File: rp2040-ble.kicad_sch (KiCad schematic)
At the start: 41 parts, among them J1 Conn_01x15, J2 Conn_01x15, J3 USB_B_Micro, J4 Conn_01x03, SW1 SW_Push, SW2 SW_Push, U1 RP2040, U2 W25Q128JVS, U3 HM-BT4502, U4 NCP1117DT33G, Y1 ABLS-12.000MHZ-B4-T

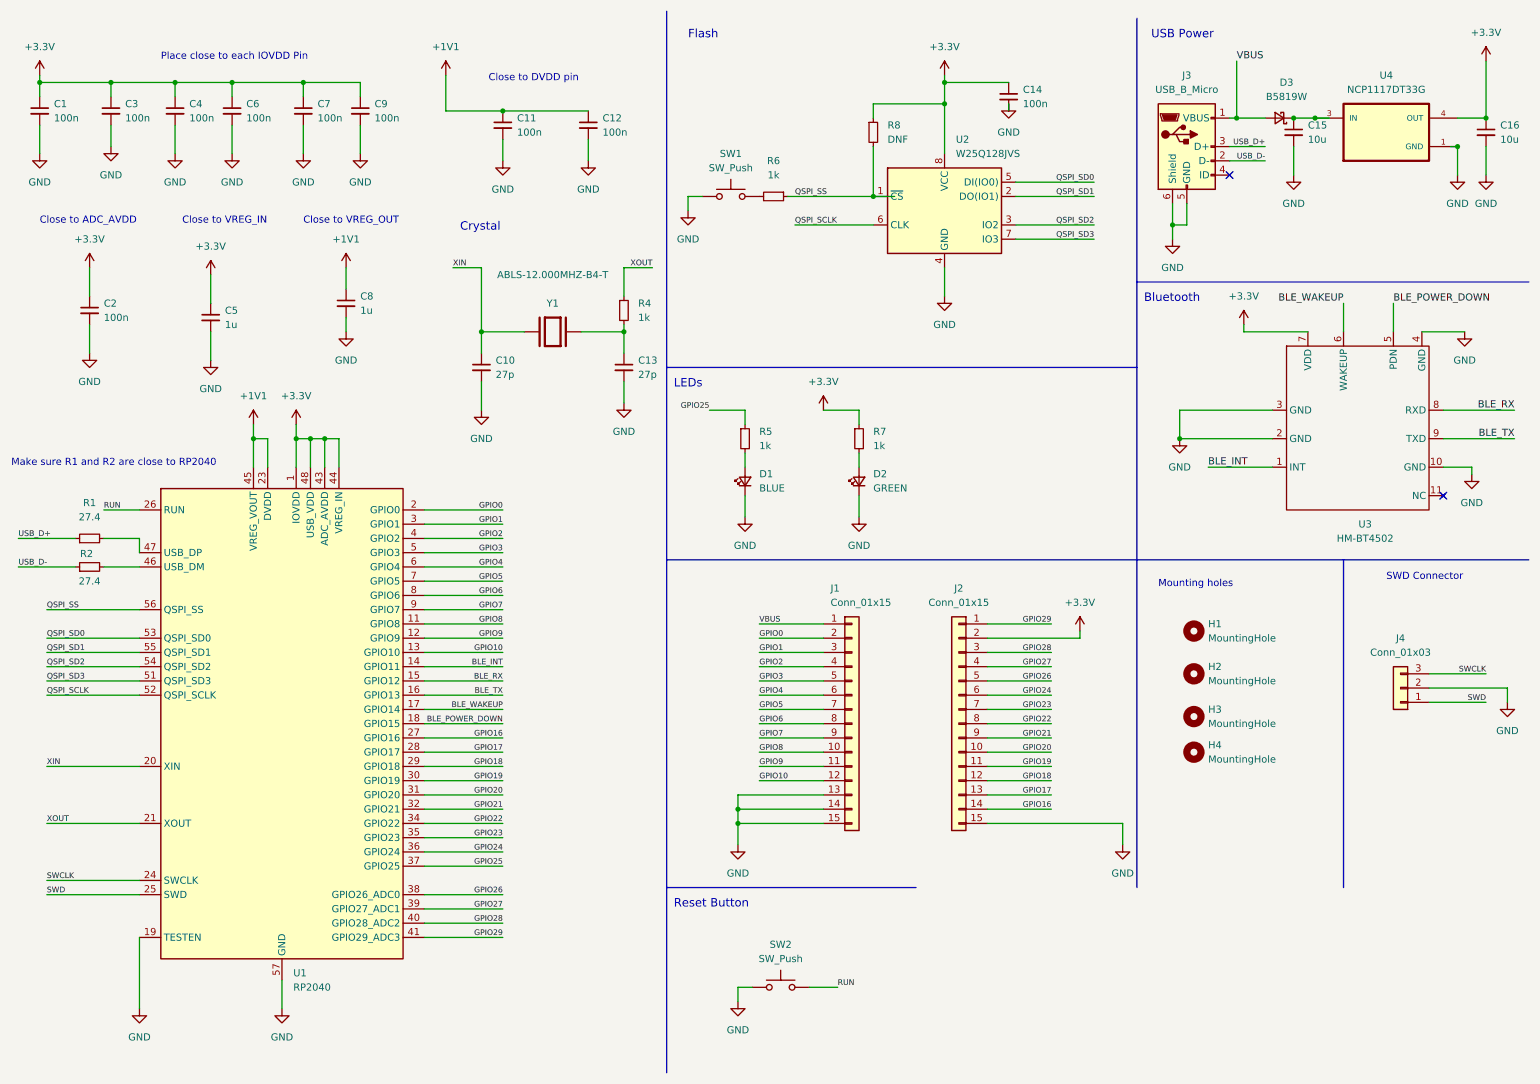
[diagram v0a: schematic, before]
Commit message: PCB roouting
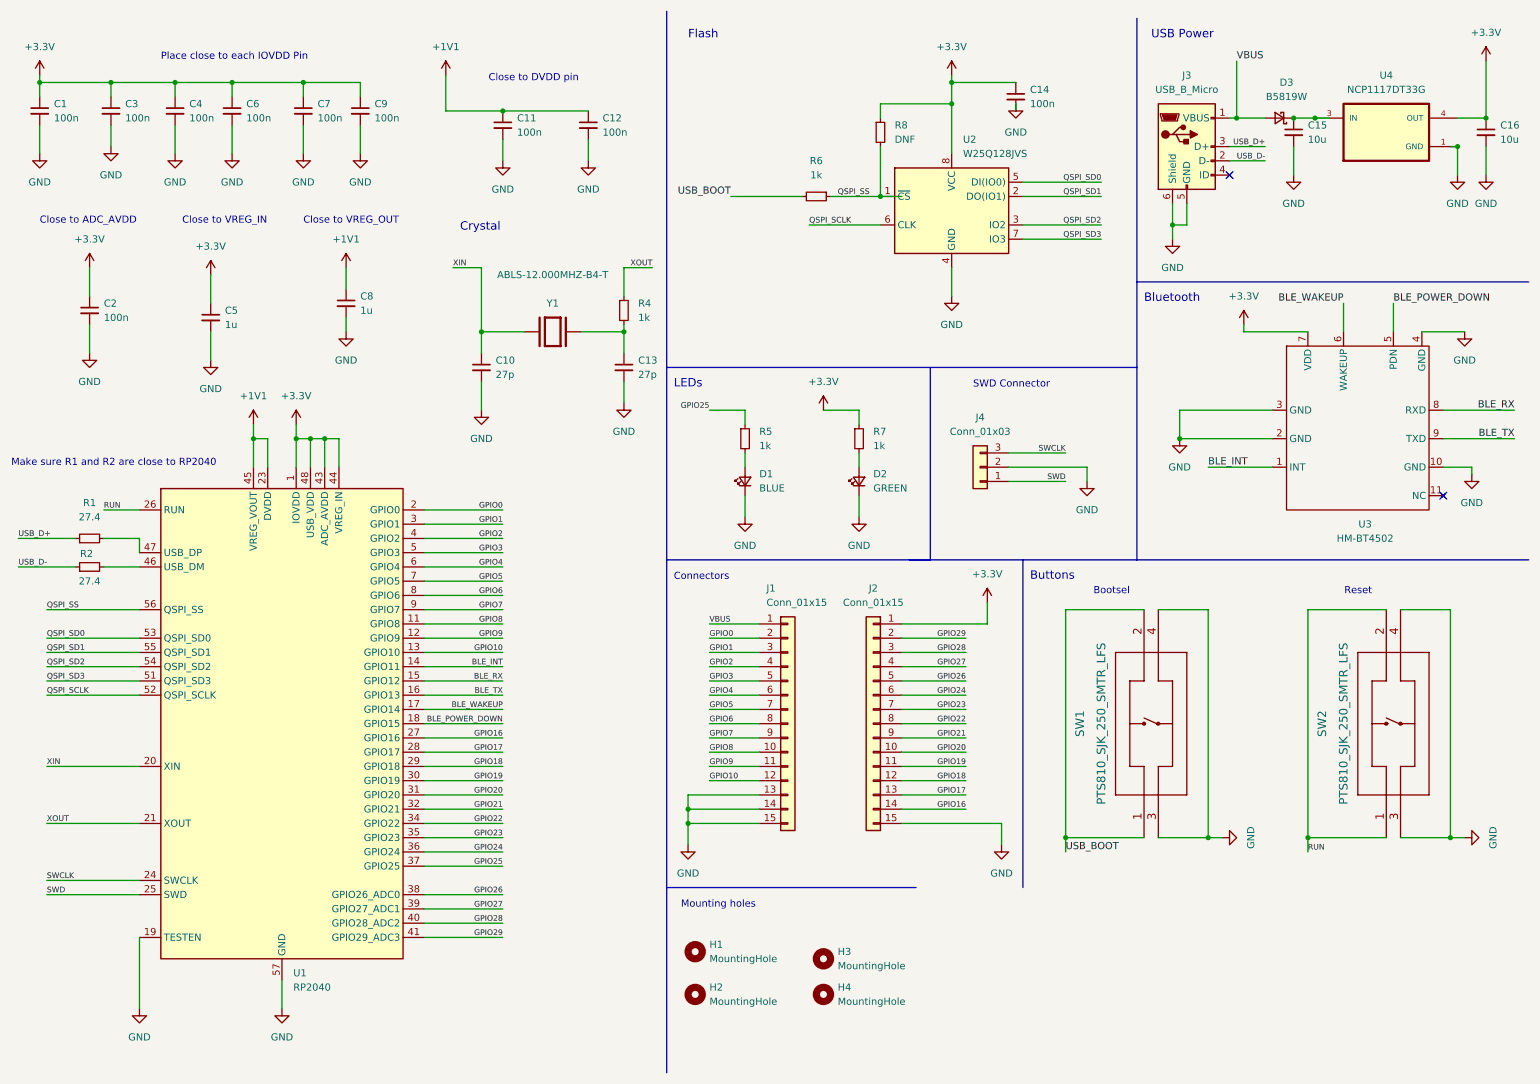
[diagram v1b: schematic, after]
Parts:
- removed SW1, SW2: SW_Push, Button_Switch_SMD:SW_SPST_B3S-1000, symbol Switch:SW_Push
- added SW1, SW2: PTS810_SJK_250_SMTR_LFS, PTS810:PTS810 SJK 250 SMTR LFS, symbol PTS810:PTS810_SJK_250_SMTR_LFS
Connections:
- net +3.3V: now also J2.1 (Pin_1); no longer J2.2 (Pin_2)
- net GND: now also SW1.3, SW1.4, SW2.3, SW2.4
- net GPIO29: now also J2.2 (Pin_2); no longer J2.1 (Pin_1)
- net RUN: now also SW2.1, SW2.2
- net USB_BOOT: now reaches R6.2
- net USB_BOOT: now also SW1.1, SW1.2
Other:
- note added: "Bootsel"
- note added: "Buttons"
- note added: "Connectors"
- note added: "Reset"
- note removed: "Reset Button"
- moved on the sheet: C14, H1, H2, H3, H4, J1, J2, J4, R6, R8, U2
